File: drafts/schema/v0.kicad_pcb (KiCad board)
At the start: 2 copper layers, 36 parts, among them P1 CONN_BATT/MOT, P2 CONN_SW, P3 CONN_SERIAL, Q1 P/N_MOS, Q2 P/N_MOS, U1 WeMos_mini, U2 N9505, U3 VHN5180A-E

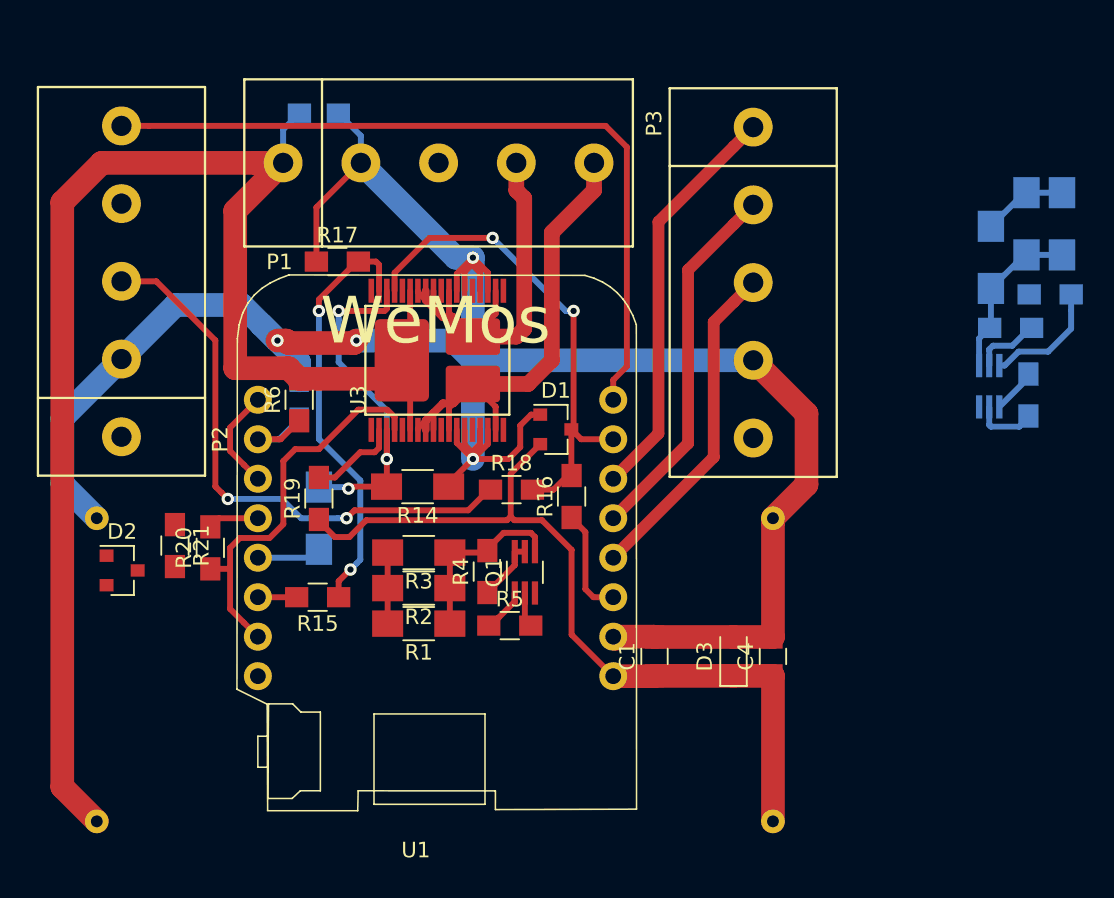
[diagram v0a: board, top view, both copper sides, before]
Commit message: routed first draft
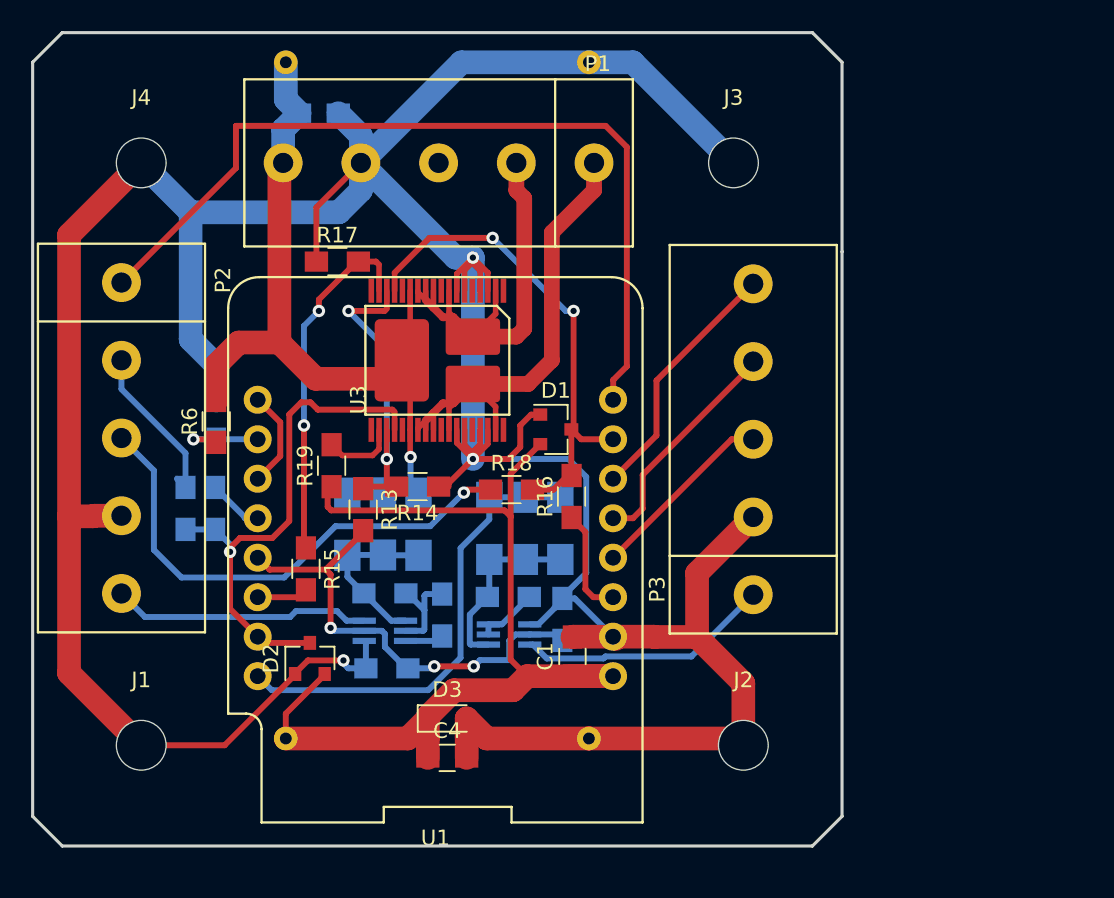
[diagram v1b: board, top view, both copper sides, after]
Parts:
- added J1: CONN_01X01, Mounting_Holes:MountingHole_3.2mm_M3, F.Cu at (114.1, 90.0)
- added J2: CONN_01X01, Mounting_Holes:MountingHole_3.2mm_M3, F.Cu at (152.9, 90.0)
- added J3: CONN_01X01, Mounting_Holes:MountingHole_3.2mm_M3, F.Cu at (152.2, 52.6)
- added J4: CONN_01X01, Mounting_Holes:MountingHole_3.2mm_M3, F.Cu at (114.1, 52.6)
- Q1, R1, R2, R20, R21, R3, R4, R5: moved to B.Cu
- R13: footprint Resistors_SMD:R_1206_HandSoldering -> Resistors_SMD:R_0805_HandSoldering; moved to F.Cu
- R14: footprint Resistors_SMD:R_1206_HandSoldering -> Resistors_SMD:R_0805_HandSoldering
- U1: footprint wemos_d1_mini:D1_mini_board -> wemos_d1_mini:Wemos-D1-mini
- moved R7 45.7 mm to (132.0, 75.8)
- moved R8 45.7 mm to (129.7, 75.8)
- moved R11 44.9 mm to (129.9, 85.1), turned to 0 degrees
- moved R9 44.8 mm to (127.4, 75.8)
- moved R12 44.2 mm to (133.5, 81.7), turned to 90 degrees
- moved R10 43.7 mm to (129.8, 80.3)
- moved Q2 41.9 mm to (129.8, 82.7), turned to 0 degrees
- moved C4 21.9 mm to (133.8, 90.9), turned to 0 degrees
- moved D3 18.8 mm to (133.8, 88.3), turned to 0 degrees
- moved U2 15.0 mm to (133.2, 70.4), turned to 270 degrees
- moved D2 13.3 mm to (125.0, 84.5), turned to 90 degrees
- moved R1 11.0 mm to (141.1, 76.1), turned to 90 degrees
- moved P2 10.1 mm to (112.8, 70.3), turned to 270 degrees
- moved P3 10.1 mm to (153.5, 70.4), turned to 90 degrees
- moved R2 7.83 mm to (138.8, 76.1), turned to 90 degrees
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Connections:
- P1 pad 1: /BATT+ -> /MOT_B
- P1 pad 2: GND -> /MOT_A
- P1 pad 4: /MOT_A -> GND
- P1 pad 5: /MOT_B -> /BATT+
- P2 pad 1: /SW_V+ -> /TX
- P2 pad 2: GND -> /SWITCH_B
- P2 pad 4: /SWITCH_B -> GND
- P2 pad 5: /TX -> /SW_V+
- P3 pad 1: /SCL -> /SER_3V3
- P3 pad 2: /SDA -> GND
- P3 pad 4: GND -> /SDA
- P3 pad 5: /SER_3V3 -> /SCL
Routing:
- net GND: track 158.9 -> 254.5 mm, vias 4 -> 3
- net /BATT+: track 101.2 -> 53.6 mm, vias 0 -> 1
- net /3V3: track 4.57 -> 30.0 mm
- net /EN_DRIVER: track 10.5 -> 30.3 mm, vias 0 -> 3
- net /SW_V+: track 0.00 -> 16.7 mm
- net /SER_3V3: track 0.00 -> 16.4 mm
- net /SWITCH_B: track 0.00 -> 11.7 mm
- net /SCL: track 26.4 -> 16.3 mm
- net VCC: track 52.5 -> 62.5 mm
- net /SDA: track 23.9 -> 14.6 mm
- net /OW: track 21.4 -> 12.2 mm
- net /SW_B: track 25.4 -> 33.6 mm, vias 0 -> 1
- net /TX: track 49.7 -> 55.9 mm
- net Net-(Q2-Pad6): track 7.81 -> 2.48 mm
- net Net-(R15-Pad1): track 27.5 -> 23.5 mm
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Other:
- board outline added: 52.1 x 52.3 mm
- net class Default: clearance 0.015 -> 0.14
- rule trace_clearance: 0.015 -> 0.14
